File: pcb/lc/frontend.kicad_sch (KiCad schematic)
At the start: 34 parts, among them J1 AudioJack3_Ground_Switch, J2 AudioJack3_Ground_Switch, U4 MCP6004, U5 REF3012

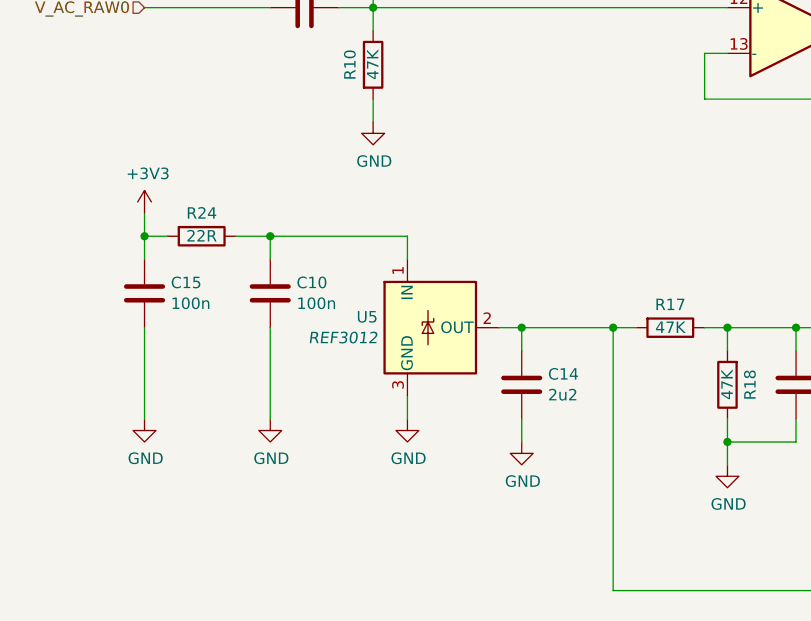
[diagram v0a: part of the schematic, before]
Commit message: * [PCB LC]
  - Change to MCP1501 reference
  - Some retouching of traces
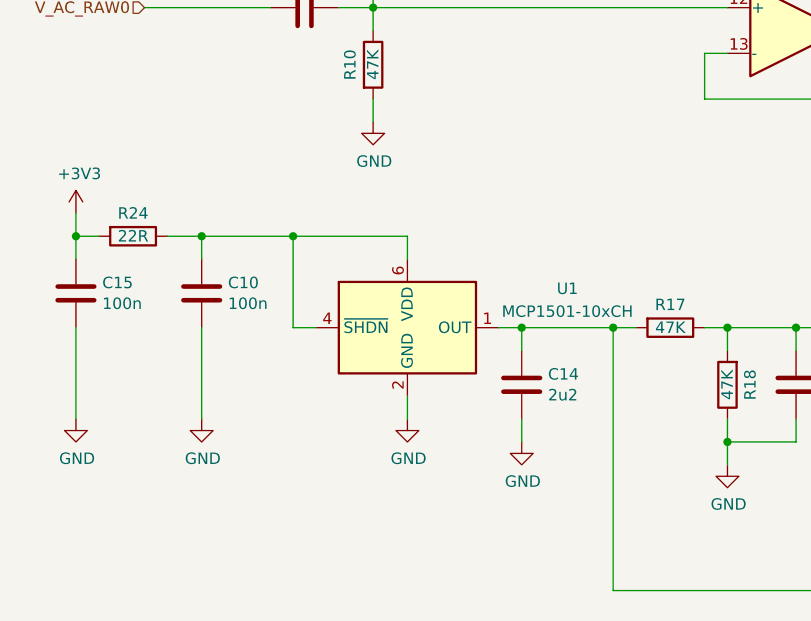
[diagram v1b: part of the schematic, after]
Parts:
- removed U5: REF3012, Package_TO_SOT_SMD:SOT-23, symbol Reference_Voltage:REF3012
- added U1: MCP1501-10xCH, Package_TO_SOT_SMD:SOT-23-6, symbol Reference_Voltage:MCP1501-10xCH
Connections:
- net GND: now also U1.2 (GND), U1.3 (GND), U1.5 (GND)
- net V_REF: now also U1.1 (OUT)
- net at C10.1, R24.1: now also U1.4 (~{SHDN}), U1.6 (VDD)
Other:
- moved on the sheet: C10, C15, R24
